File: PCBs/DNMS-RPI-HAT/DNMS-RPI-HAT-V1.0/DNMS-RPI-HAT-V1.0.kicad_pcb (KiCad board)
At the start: 2 copper layers, 65 x 30 mm, 17 parts, among them J1 Conn_02x20_Odd_Even, J2 RJ12, J3 RJ12, J4 Conn_01x05, J6 Conn_01x04_Male, J7 Conn_01x04_Male, J8 Screw_Terminal_01x02, U1 P82B715P, U2 P82B715DR

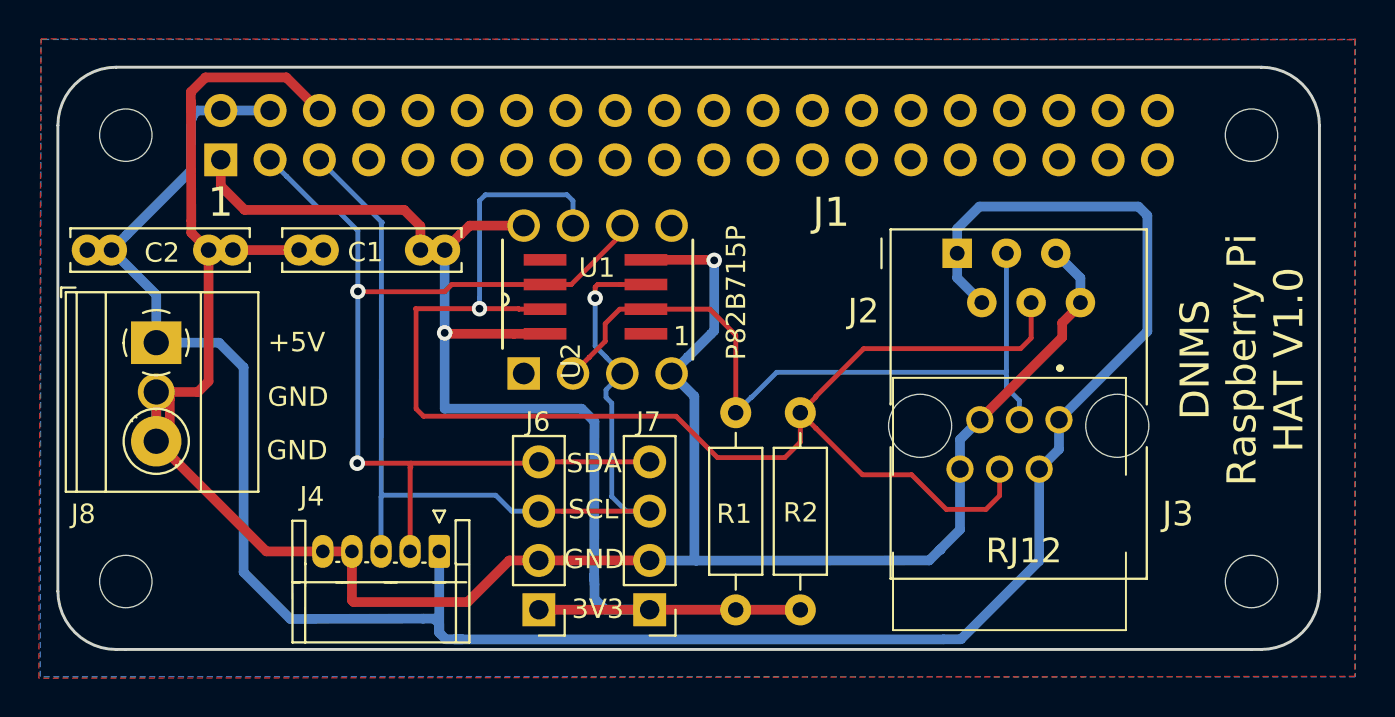
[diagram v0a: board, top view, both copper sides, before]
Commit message: new firmware
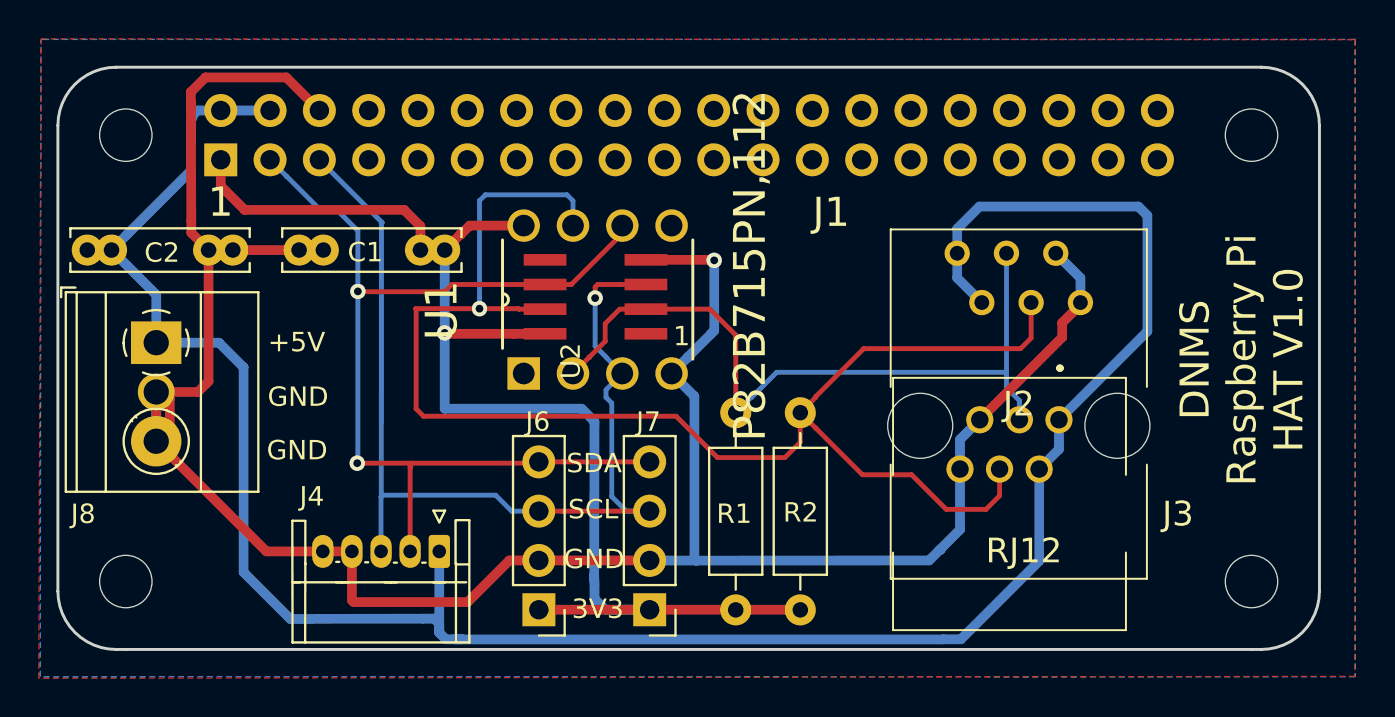
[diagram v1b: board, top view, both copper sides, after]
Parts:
- J2: footprint Connector_RJ:RJ12_Amphenol_54601 -> 54601906WPLF:54601906WPLF
- J6, J7: value Conn_01x04_Male -> Conn_01x04_Pin
- U1: value P82B715P -> P82B715PN,112; footprint P82B715:DIP254P762X420-8 -> P82B715:P82B715 DIP8
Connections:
- J1 pad 10: Net-(J1-Pad10) -> unconnected-(J1-Pin_10-Pad10)
- J1 pad 11: Net-(J1-Pad11) -> unconnected-(J1-Pin_11-Pad11)
- J1 pad 12: Net-(J1-Pad12) -> unconnected-(J1-Pin_12-Pad12)
- J1 pad 13: Net-(J1-Pad13) -> unconnected-(J1-Pin_13-Pad13)
- J1 pad 14: Net-(J1-Pad14) -> unconnected-(J1-Pin_14-Pad14)
- J1 pad 15: Net-(J1-Pad15) -> unconnected-(J1-Pin_15-Pad15)
- J1 pad 16: Net-(J1-Pad16) -> unconnected-(J1-Pin_16-Pad16)
- J1 pad 17: Net-(J1-Pad17) -> unconnected-(J1-Pin_17-Pad17)
- J1 pad 18: Net-(J1-Pad18) -> unconnected-(J1-Pin_18-Pad18)
- J1 pad 19: Net-(J1-Pad19) -> unconnected-(J1-Pin_19-Pad19)
- J1 pad 20: Net-(J1-Pad20) -> unconnected-(J1-Pin_20-Pad20)
- J1 pad 21: Net-(J1-Pad21) -> unconnected-(J1-Pin_21-Pad21)
- J1 pad 22: Net-(J1-Pad22) -> unconnected-(J1-Pin_22-Pad22)
- J1 pad 23: Net-(J1-Pad23) -> unconnected-(J1-Pin_23-Pad23)
- J1 pad 24: Net-(J1-Pad24) -> unconnected-(J1-Pin_24-Pad24)
- J1 pad 25: Net-(J1-Pad25) -> unconnected-(J1-Pin_25-Pad25)
- J1 pad 26: Net-(J1-Pad26) -> unconnected-(J1-Pin_26-Pad26)
- J1 pad 27: Net-(J1-Pad27) -> unconnected-(J1-Pin_27-Pad27)
- J1 pad 28: Net-(J1-Pad28) -> unconnected-(J1-Pin_28-Pad28)
- J1 pad 29: Net-(J1-Pad29) -> unconnected-(J1-Pin_29-Pad29)
- J1 pad 30: Net-(J1-Pad30) -> unconnected-(J1-Pin_30-Pad30)
- J1 pad 31: Net-(J1-Pad31) -> unconnected-(J1-Pin_31-Pad31)
- J1 pad 32: Net-(J1-Pad32) -> unconnected-(J1-Pin_32-Pad32)
- J1 pad 33: Net-(J1-Pad33) -> unconnected-(J1-Pin_33-Pad33)
- J1 pad 34: Net-(J1-Pad34) -> unconnected-(J1-Pin_34-Pad34)
- J1 pad 35: Net-(J1-Pad35) -> unconnected-(J1-Pin_35-Pad35)
- J1 pad 36: Net-(J1-Pad36) -> unconnected-(J1-Pin_36-Pad36)
- J1 pad 37: Net-(J1-Pad37) -> unconnected-(J1-Pin_37-Pad37)
- J1 pad 38: Net-(J1-Pad38) -> unconnected-(J1-Pin_38-Pad38)
- J1 pad 39: Net-(J1-Pad39) -> unconnected-(J1-Pin_39-Pad39)
- J1 pad 40: Net-(J1-Pad40) -> unconnected-(J1-Pin_40-Pad40)
- J1 pad 7: Net-(J1-Pad7) -> unconnected-(J1-Pin_7-Pad7)
- J1 pad 8: Net-(J1-Pad8) -> unconnected-(J1-Pin_8-Pad8)
- J1 pad 9: Net-(J1-Pad9) -> unconnected-(J1-Pin_9-Pad9)
- U1 pad 1: Net-(U1-Pad1) -> unconnected-(U1-N.C._2-Pad1)
- U1 pad 5: Net-(U1-Pad5) -> unconnected-(U1-N.C.-Pad5)
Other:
- net class Default removed
- rule pad_to_mask_clearance: 0.051 -> 0
